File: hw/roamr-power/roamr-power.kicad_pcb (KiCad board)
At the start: 2 copper layers, 8.7 x 4.4 mm, 45 parts, among them J1 Conn_01x02_Socket, J2 Conn_01x02_Socket, J3 Conn_01x02_Socket, P2 USB_C_Plug_USB2.0, Q1 Q_PMOS_DSG, SW1 SW_SPDT, U1 TPS56A37RPAR, U2 TPS2553DDBVR

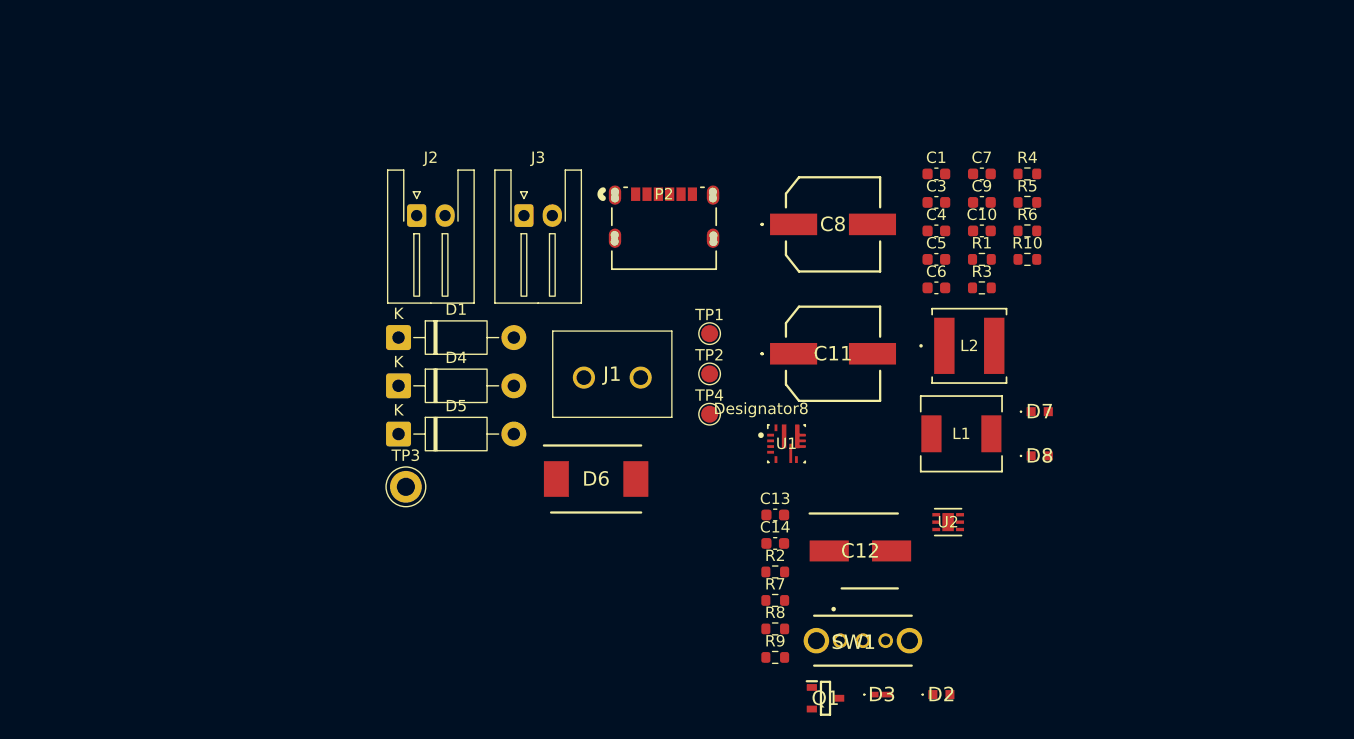
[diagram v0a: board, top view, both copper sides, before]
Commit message: layout
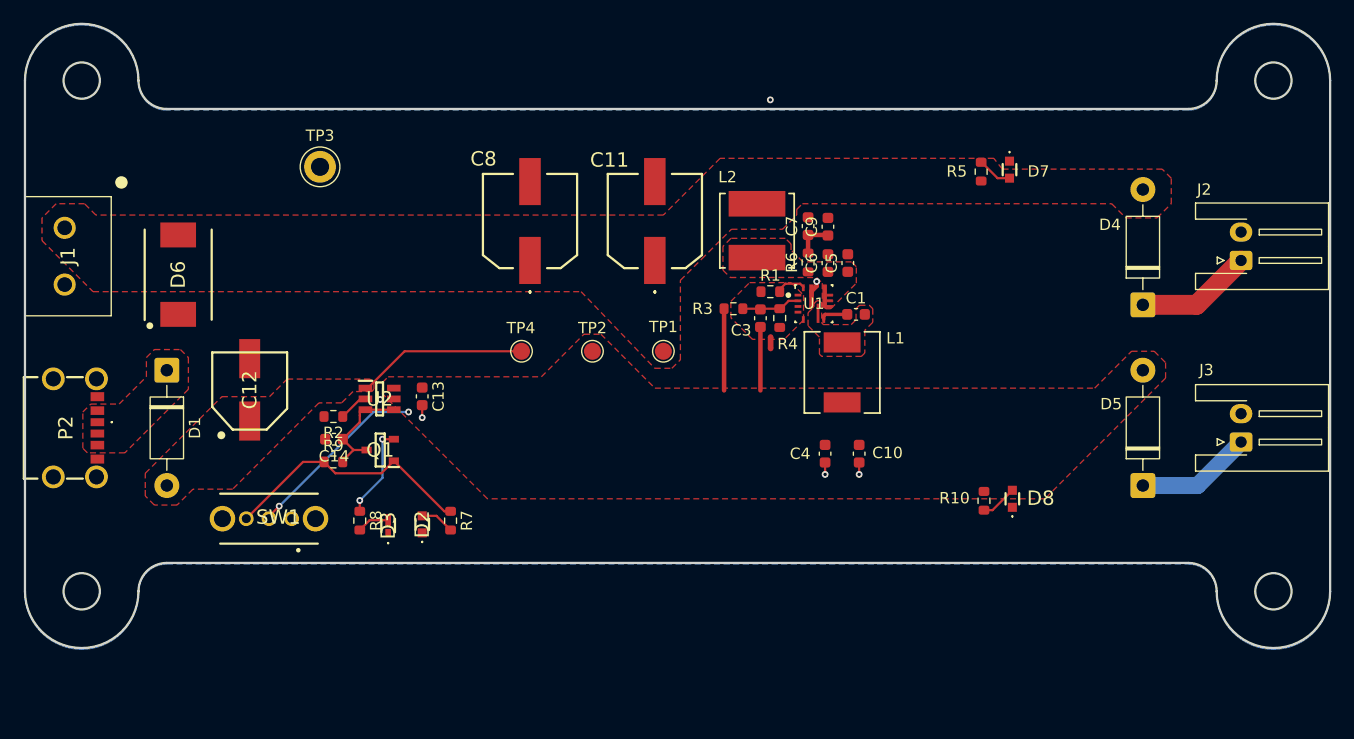
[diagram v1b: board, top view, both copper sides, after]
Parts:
- added NT1: NetTie_2, NetTie:NetTie-2_SMD_Pad0.5mm, F.Cu at (134.7, 71.0)
- L2: footprint VLS6045EX_4R7M:IND_VLS6045EX-4R7M_TDK-L -> VLS6045EX_4R7M:IND_VLS6045EX-4R7M_TDK
- P2: footprint USB4125-GF-A:CONN6_USB4125_GCT -> USB4125-GF-A:USB4125GFA
- U2: footprint TPS2553DDBVR:DRV6_1P6X1_TEX -> TPS2553DDBVR:SOT95P280X145-6N
- moved J2 72.7 mm to (176.2, 63.8), turned to 90 degrees
- moved J3 66.3 mm to (176.2, 79.8), turned to 90 degrees
- moved D4 66.0 mm to (167.5, 67.7), turned to 90 degrees
- moved D5 65.7 mm to (167.5, 83.6), turned to 90 degrees
- moved C12 55.7 mm to (88.8, 75.2), turned to 90 degrees
- moved P2 55.6 mm to (72.6, 78.5), turned to -90 degrees
- moved SW1 53.4 mm to (90.5, 86.5), turned to 180 degrees
- moved U2 51.3 mm to (100.2, 76.0)
- moved D2 48.1 mm to (104.0, 87.0), turned to 90 degrees
- moved J1 47.6 mm to (72.5, 60.9), turned to -90 degrees
- moved D3 46.0 mm to (101.0, 87.1), turned to 90 degrees
- moved Q1 44.9 mm to (100.3, 80.5), turned to 180 degrees
- moved R9 42.6 mm to (96.2, 81.5)
- moved R2 41.3 mm to (96.2, 77.5), turned to 180 degrees
- moved D6 41.0 mm to (82.5, 65.0), turned to 90 degrees
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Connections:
- net Net-(D1-K) renamed /USB_OUT
- net Net-(D4-K) renamed /12V_OUT
- net Net-(D5-K) renamed /5V_OUT
- net Net-(U1-SW) renamed /12V to 5V/SW_OUT
- net Net-(U1-VIN) renamed /12V to 5V/12V_SW
- C10 pad 1: Net-(C10-Pad1) -> +5V
- C11 pad 1: Net-(C11-Pad1) -> +12V
- C4 pad 2: Net-(C10-Pad1) -> GND
- C7 pad 2: Net-(C7-Pad2) -> GND
- C8 pad 2: Net-(C11-Pad1) -> GND
- C9 pad 1: Net-(C7-Pad2) -> Net-(C7-Pad1)
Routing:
- net /Phone Charging/CHG_EN: track 0.00 -> 22.8 mm
- net +5V: track 0.00 -> 16.3 mm, vias 0 -> 2
- net VCTRL_5V: track 0.00 -> 15.1 mm
- net /12V_OUT: track 0.00 -> 10.3 mm
- net /5V_OUT: track 0.00 -> 10.2 mm
- net Net-(Q1-S): track 0.00 -> 6.23 mm, vias 0 -> 2
- net /Phone Charging/CURR_LIM_nFLT: track 0.00 -> 5.21 mm
- net GND: track 0.00 -> 4.70 mm, vias 0 -> 5
- net Net-(D8-A): track 0.00 -> 3.22 mm
- net Net-(D7-A): track 0.00 -> 3.08 mm
- net Net-(D2-A): track 0.00 -> 3.02 mm
- net Net-(D3-A): track 0.00 -> 2.86 mm
- net Net-(U2-ILIM): track 0.00 -> 2.64 mm
- net Net-(U1-BOOT): track 0.00 -> 2.46 mm
- net Net-(U1-FB): track 0.00 -> 1.90 mm
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- added copper zone on F.Cu, net +12V
- added copper zone on F.Cu, net +5V
- added copper zone on F.Cu, net /12V to 5V/12V_SW
- added copper zone on F.Cu, net /12V to 5V/SW_OUT
- added copper zone on F.Cu, net /USB_OUT
- added copper zone on B.Cu, net GND
- added copper zone on F.Cu, net GND
- added copper zone on F.Cu, net GNDA
- added copper zone on F.Cu, net VCTRL_5V
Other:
- board size 8.7 x 4.4 mm -> 115 x 55 mm
